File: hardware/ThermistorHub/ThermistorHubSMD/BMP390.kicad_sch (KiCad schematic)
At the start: 5 parts

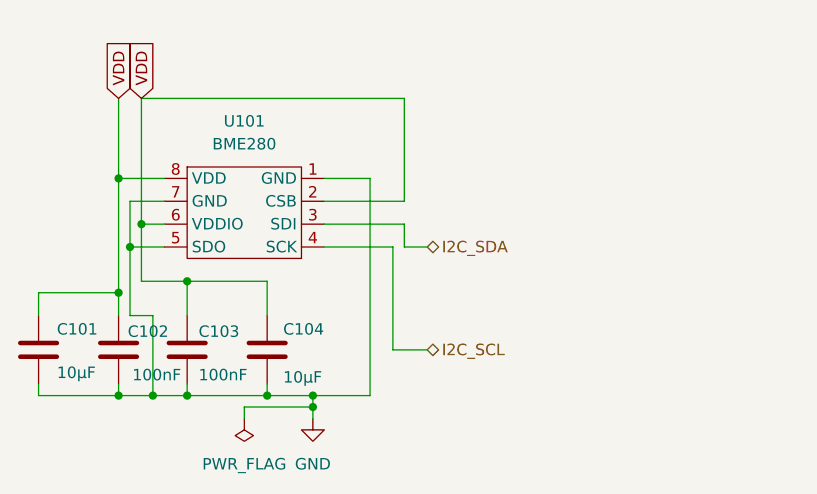
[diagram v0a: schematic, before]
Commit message: 途中まで
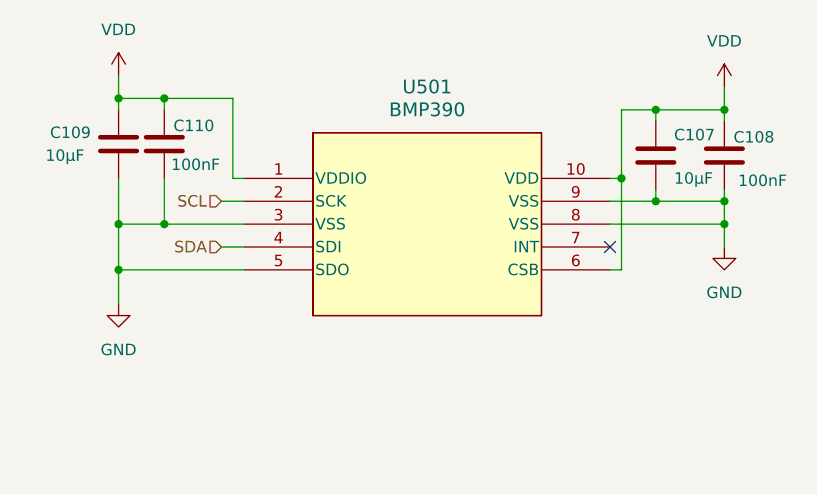
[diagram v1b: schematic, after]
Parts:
- removed C101, C104: 10μF, Capacitor_SMD:C_0603_1608Metric, symbol Device:C
- removed C102, C103: 100nF, Capacitor_SMD:C_0402_1005Metric, symbol Device:C
- removed U101: (no value), WOBCLibrary:BME280, symbol WOBCLibrary:BME280
- added C107, C109: 10μF, Capacitor_SMD:C_0603_1608Metric, symbol Device:C
- added C108, C110: 100nF, Capacitor_SMD:C_0402_1005Metric, symbol Device:C
- added U501: BMP390, Library:10LGA_2X2X0p75_BOS, symbol New_Library_0:BMP390
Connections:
- net GND: now also C107.2, C108.2, C109.2, C110.2, U501.3 (VSS), U501.5 (SDO), U501.8 (VSS), U501.9 (VSS)
- net VDD: now also C107.1, C108.1, C109.1, C110.1, U501.1 (VDDIO), U501.10 (VDD), U501.6 (CSB)
- new net SCL: U501.2 (SCK)
- new net SDA: U501.4 (SDI)
- no-connect marks 0 -> 1
